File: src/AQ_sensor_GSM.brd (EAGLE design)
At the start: 110.2 x 66.3 mm, 177 parts, among them J1 F-1X03-SIP-100-32, J2 53261-0871, J4 S8411-45R, Q2 MMBT2222, Q3 MMBT2222, Q4 MMBT2222, Q5 MMBT2222, Q6 MMBT2222, Q7 MMBT2222, Q8 FS8205, T1 S8050, T2 S8050, U1 CP2102N-A02-GQFN28, U2 DS1307Z, U3 TP4056, U4 TPS63802DLAR, U5 TXS0108EPWR, U6 TPS63802DLAR, X1 ESP32-S3-WROOM-1-N16R8, Y1 32.768kHz

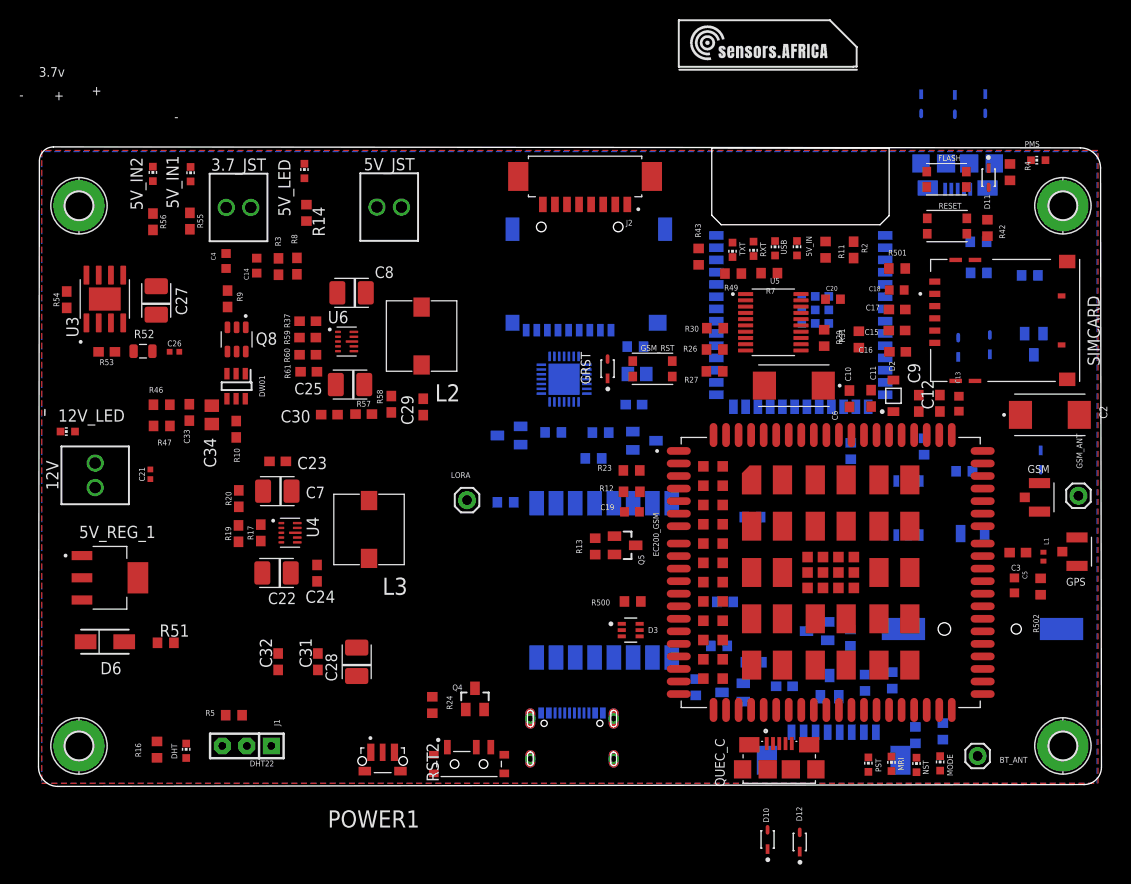
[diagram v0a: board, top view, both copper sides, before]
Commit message: Routing in Progress
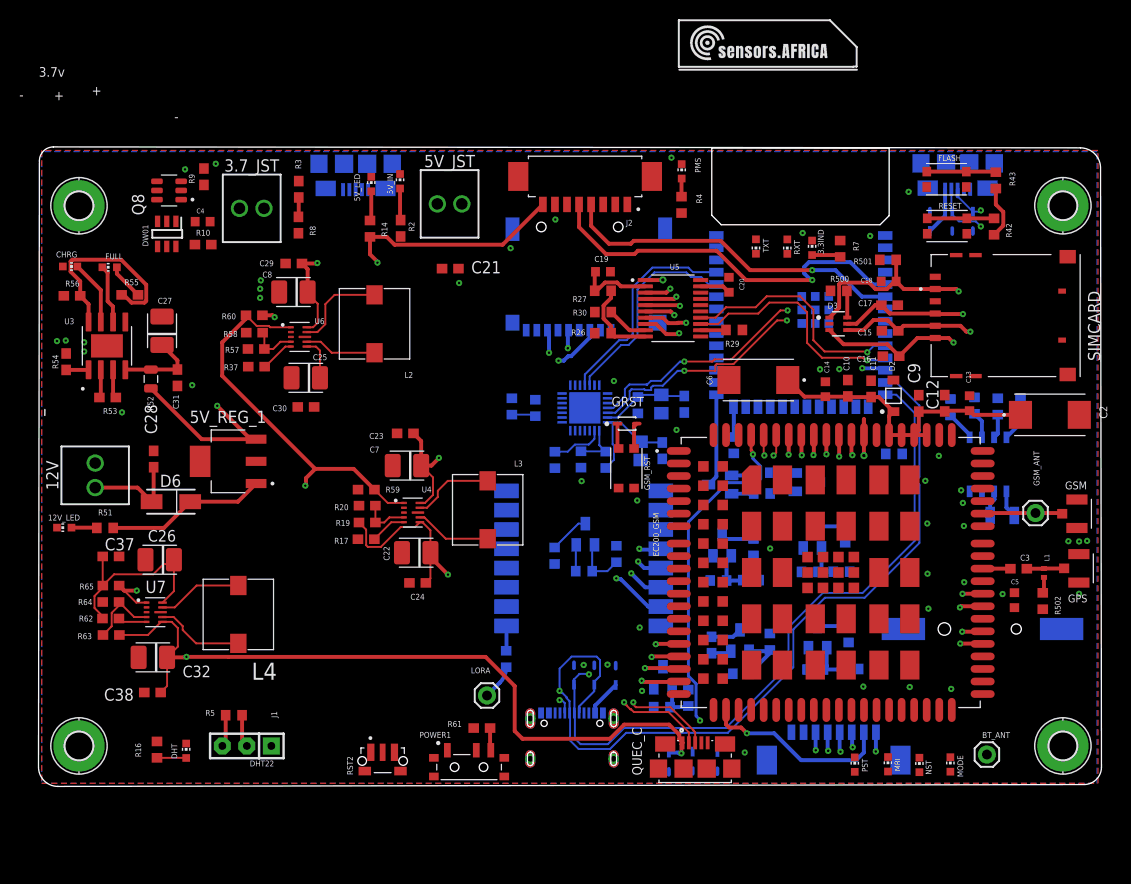
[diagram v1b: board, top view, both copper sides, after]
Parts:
- removed 5V_IN1, 5V_IN2: ORANGE, led:CHIP-LED0603
- removed R40: 10K, rcl:R0603
- removed USB: (no value), led:CHIP-LED0603
- added 3.3IND: (no value), led:CHIP-LED0603
- added C37, C38: 0.1uF, rcl:C0603
- added CHRG, FULL: ORANGE, led:CHIP-LED0603
- added L4: 784778010, Fixed Inductors:784778010
- added POWER: 10118192-0001LF, AQ_sensor_GSM:AMPHENOL_10118192-0001LF
- added R62: 100k, SparkFun-Resistors:0603
- added R63: 432k, SparkFun-Resistors:0603
- added R64: 47k, SparkFun-Resistors:0603
- added R65: 1k, SparkFun-Resistors:0603
- added R66, R67: 10K, rcl:R0603
- added U7: TPS63802DLAR, TPS63802DLAR:VREG_TPS63802DLAR
- C21: device SparkFun-Capacitors:0402-TIGHT -> rcl:C0603
- C26: value 22pF -> TAJB106K016RNJ; device SparkFun-Capacitors:0402-TIGHT -> Resistor_Capacitor:CAP_TANT_B
- C28: value TAJB106K016RNJ -> 22pF; device Resistor_Capacitor:CAP_TANT_B -> rcl:C0603
- C32: value 0.1uF -> TAJB106K016RNJ; device rcl:C0603 -> Resistor_Capacitor:CAP_TANT_B
- moved D11 67.8 mm to (68.3, -0.88), flipped to the bottom
- moved C14 60.3 mm to (82.1, 37.7), turned to 270 degrees
- moved D4 53.3 mm to (56.0, 8.07), turned to 90 degrees
- moved D9 51.8 mm to (60.3, 8.03)
- moved R22 51.0 mm to (73.3, 8.19), turned to 180 degrees
- moved D8 50.8 mm to (58.1, 8.06)
- moved C33 49.2 mm to (65.2, 31.3), flipped to the bottom
- moved R2 47.0 mm to (38.0, 54.4)
- moved R46 46.4 mm to (59.3, 30.4), flipped to the bottom, turned to 90 degrees
- moved C34 44.6 mm to (62.9, 31.3), flipped to the bottom
- moved R21 43.9 mm to (76.3, 11.5), turned to 270 degrees
- moved R47 43.6 mm to (56.7, 30.4), flipped to the bottom, turned to 270 degrees
- moved Q3 43.3 mm to (73.2, 11.6), turned to 0 degrees
- moved R28 41.8 mm to (54.0, 20.4)
- moved 5V_IN 41.7 mm to (38.0, 59.2)
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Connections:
- removed net IO15: R40.1, X1.8
- removed net IO5: X1.5
- removed net IO6: X1.6
- removed net IO7: X1.7
- removed net IO8: X1.12
- removed net LBV: R10.2
- removed net L_MIS0: U$1.13, X1.38
- removed net L_MOSI: U$1.14, X1.39
- removed net L_SCK: U$1.12, X1.15
- removed net SD_CLK: MICRO_SD1.5, X1.31
- removed net SD_MISO: MICRO_SD1.3, X1.34
- removed net SD_MOSI: MICRO_SD1.7, X1.33
- new net IO21: X1.23
- new net IO35: X1.28
- new net IO36: X1.29
- new net IO37: X1.30
- new net IO38: X1.31
- new net IO40: X1.33
- new net IO41: X1.34
- new net IO42: X1.35
- new net IO45: R66.1, X1.26
- new net IO46: R67.1, X1.16
- new net MISO: MICRO_SD1.3, U$1.13, X1.38
- new net MOSI: MICRO_SD1.7, U$1.14, X1.39
- new net N$149: L4.2, U7.9
- new net N$150: L4.1, U7.7
- new net N$151: R62.1, U7.5
- new net N$152: R63.2, R64.1, U7.4
- new net SPI_CLK: MICRO_SD1.5, U$1.12, X1.15
- net 12V-IN: now also C26.1, C28.1, C37.1, R62.2, R65.2, U7.10; no longer C21.1
- net 4.0V_OUT: now also C10.1, C11.1, C12.1, C13.2, C14.2, C2.1, C5.2, C6.1, C9.1, D2.1, EC200_GSM.57, EC200_GSM.58, EC200_GSM.59, EC200_GSM.60, MODE.A, MRI.A, NST.A, PST.A, R502.2
- net BOOST_EN: now also R65.1, U7.1
- net DHT_LED: no longer X1.30
- net DHT_OUT: now also X1.7; no longer X1.29
- net GND: now also 3.3IND.C, C37.2, C38.2, POWER.4, POWER.5, POWER.SH1, POWER.SH2, POWER.SH3, POWER.SH4, POWER.SH5, POWER.SH6, R64.2, R66.2, R67.2, U7.2, U7.3, U7.8; no longer R40.2, USB.C
- net GSM_RST_O: now also X1.8; no longer X1.35
- net L_NSS: now also X1.12; no longer X1.16
- net N$138: no longer C28.1, C32.1
- net N$143: now also FULL.A; no longer 5V_IN1.A
- net N$145: now also CHRG.A; no longer 5V_IN2.A
- net N$146: now also FULL.C; no longer 5V_IN1.C
- net N$147: now also CHRG.C; no longer 5V_IN2.C
- net N$38: now also 3.3IND.A; no longer USB.A
- net PMS_LED: no longer X1.28
- net PMS_RX: now also X1.5; no longer X1.23
- net PMS_TX: now also X1.6; no longer X1.26
- net VUSB: now also C21.1, C32.1, C38.1, POWER.1, R63.1, U7.6; no longer C26.1
- net V_LIPO: now also R10.2; no longer C10.1, C11.1, C12.1, C13.2, C14.2, C2.1, C5.2, C6.1, C9.1, D2.1, EC200_GSM.57, EC200_GSM.58, EC200_GSM.59, EC200_GSM.60, MODE.A, MRI.A, NST.A, PST.A, R502.2
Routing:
- net VUSB: track 0.00 -> 173.8 mm, vias 0 -> 3
- net 5V_OUT: track 0.00 -> 89.5 mm, vias 0 -> 2
- net EUSB_N: track 0.00 -> 85.6 mm, vias 0 -> 1
- net USIM_VDD: track 0.00 -> 83.7 mm, vias 0 -> 2
- net SIMRST: track 0.00 -> 78.8 mm, vias 0 -> 2
- net EUSB_P: track 0.00 -> 78.0 mm, vias 0 -> 2
- net SIMCLK: track 0.00 -> 77.0 mm, vias 0 -> 2
- net SIMDATA: track 0.00 -> 75.3 mm, vias 0 -> 2
- net L_NSS: track 0.00 -> 68.8 mm, vias 0 -> 2
- net BOOST_EN: track 0.00 -> 66.9 mm, vias 0 -> 2
- net G_USB_VBUS: track 0.00 -> 57.7 mm, vias 0 -> 3
- net EUART_N: track 0.00 -> 53.9 mm, vias 0 -> 3
- net EUART_P: track 0.00 -> 51.5 mm, vias 0 -> 3
- net G_USB_N: track 0.00 -> 42.9 mm, vias 0 -> 2
- net G_USB_P: track 0.00 -> 42.9 mm, vias 0 -> 2
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
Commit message: 90% routed
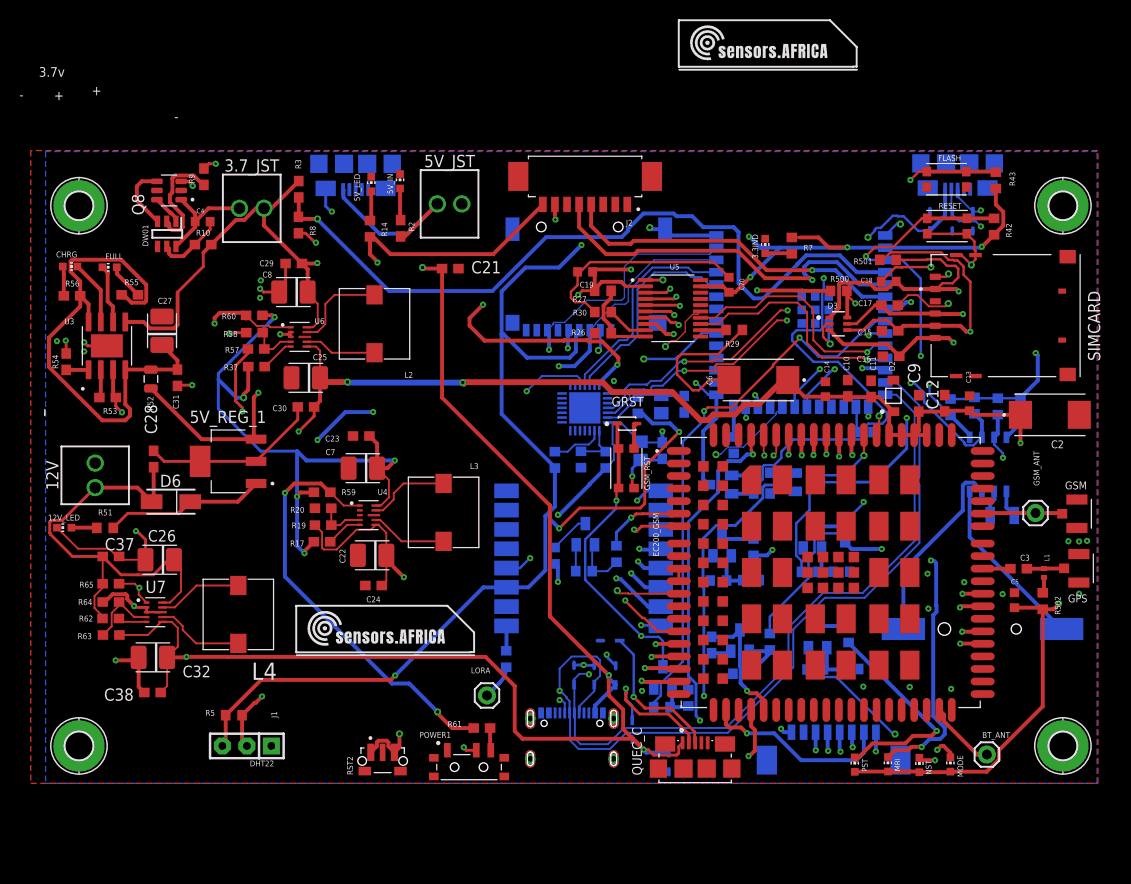
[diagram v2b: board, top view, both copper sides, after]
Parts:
- removed DHT: GREEN, led:CHIP-LED0603
- removed PMS: ORANGE, led:CHIP-LED0603
- removed R11, R49: 200, rcl:R0603
- removed R16, R4: 470R, rcl:R0603
- removed RXT, TXT: (no value), led:CHIP-LED0603
- moved D10 16.8 mm to (59.8, 11.6), turned to 0 degrees
- moved D11 7.06 mm to (62.1, 2.37)
- moved R7 5.02 mm to (78.6, 52.6)
- moved 3.3IND 4.86 mm to (75.8, 52.5)
- moved C23 4.58 mm to (34.0, 32.8)
- moved C24 4.58 mm to (35.2, 17.3)
- moved C7 4.58 mm to (34.1, 29.5)
- moved L3 4.58 mm to (42.5, 24.9)
- moved R17 4.58 mm to (29.9, 21.9)
- moved U4 4.58 mm to (34.7, 24.6)
- moved R19 4.58 mm to (30.0, 23.6)
- moved R20 4.58 mm to (30.0, 25.4)
- moved R59 4.58 mm to (29.9, 27.0)
- moved C22 4.58 mm to (35.1, 20.5)
- moved R67 3.78 mm to (86.2, 33.2)
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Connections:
- removed net DHT_LED: R16.2
- removed net N$54 (its old number): R11.1, TXT.C
- removed net N$55 (its old number): R49.1, RXT.C
- removed net N$56 (its old number): TXT.A, U1.19
- removed net N$57 (its old number): RXT.A, U1.18
- removed net PMS_LED: R4.2
- net +3V3: no longer R11.2, R49.2
- net GND: no longer DHT.C, PMS.C, RST2.S1, RST2.S2
- net N$27: now also U1.18; no longer DHT.A, R16.1
- net N$4: now also U1.19; no longer PMS.A, R4.1
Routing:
- net ESP_RST: track 6.93 -> 193.8 mm, vias 0 -> 4
- net +3V3: track 14.5 -> 188.4 mm, vias 0 -> 8
- net GND: track 10.5 -> 171.0 mm, vias 47 -> 44
- net DHT_OUT: track 3.39 -> 136.9 mm, vias 0 -> 4
- net 4.0V_OUT: track 36.6 -> 169.2 mm, vias 0 -> 6
- net 5V_OUT: track 89.5 -> 219.8 mm, vias 2 -> 6
- net VUSB: track 173.8 -> 278.8 mm, vias 3 -> 6
- net DTR: track 2.30 -> 107.1 mm, vias 0 -> 3
- net V_LIPO: track 23.1 -> 111.6 mm, vias 3 -> 6
- net RTS: track 2.66 -> 84.7 mm, vias 0 -> 2
- net BMSV: track 2.02 -> 78.8 mm, vias 0 -> 1
- net USIM_GND: track 0.00 -> 76.8 mm, vias 0 -> 2
- net VDD_EXT: track 7.77 -> 68.6 mm, vias 0 -> 4
- net GSM_RST_O: track 0.00 -> 57.3 mm, vias 0 -> 2
- net N$34: track 0.00 -> 55.7 mm, vias 0 -> 2
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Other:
- board size 110.2 x 66.3 mm -> 9.2 x 5.7 mm
